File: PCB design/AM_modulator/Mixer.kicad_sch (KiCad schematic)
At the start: 8 parts

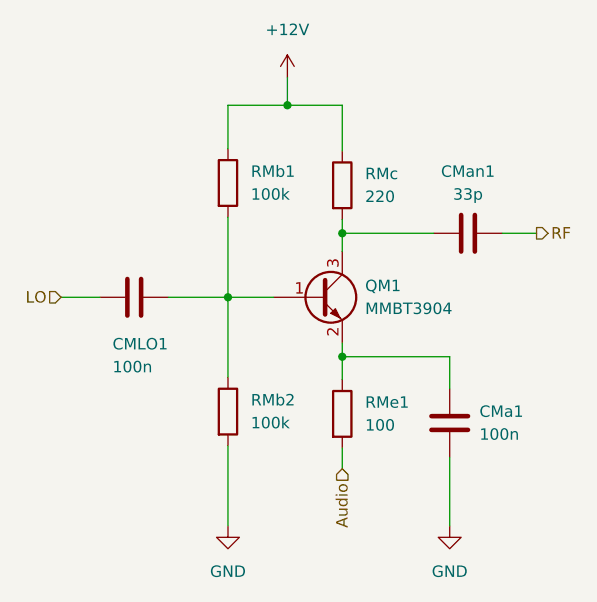
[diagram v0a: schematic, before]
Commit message: Avances placa
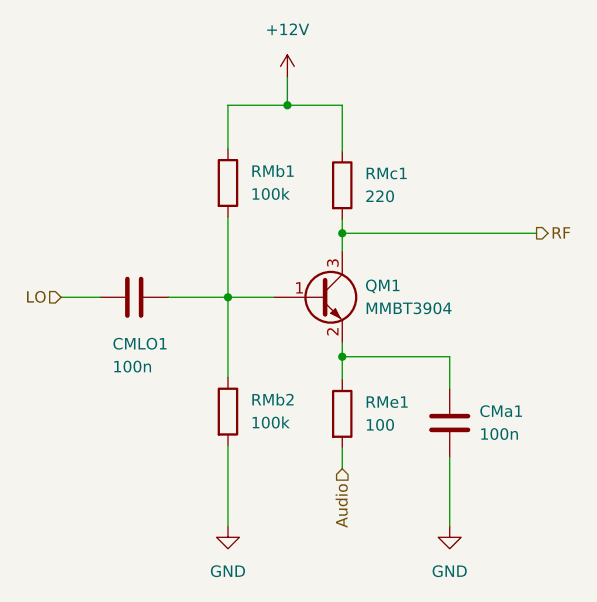
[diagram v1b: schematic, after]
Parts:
- removed CMan1: 33p, Capacitor_SMD:C_0805_2012Metric_Pad1.18x1.45mm_HandSolder, symbol Device:C
- renumbered RMc to RMc1
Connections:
- net RF: now also QM1.3 (C), RMc1.2
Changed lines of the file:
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@@
-    (stroke (width 0) (type default) (color 0 0 0 0))
-  )
-  (wire (pts (xy 156.972 81.788) (xy 160.782 81.788))
     (stroke (width 0) (type default) (color 0 0 0 0))
   )
@@
     (stroke (width 0) (type default) (color 0 0 0 0))
   )
-  (wire (pts (xy 139.192 81.788) (xy 149.352 81.788))
+  (wire (pts (xy 139.192 81.788) (xy 160.782 81.788))
     (stroke (width 0) (type default) (color 0 0 0 0))
   )
@@
     (pin "2")
   )
-  (symbol (lib_id "Device:C") (at 153.162 81.788 90) (unit 1)
-    (in_bom yes) (on_board yes) (fields_autoplaced)
-    (property "Reference" "CMan1" (id 0) (at 153.162 74.93 90))
-    (property "Value" "33p" (id 1) (at 153.162 77.47 90))
-    (property "Footprint" "Capacitor_SMD:C_0805_2012Metric_Pad1.18x1.45mm_HandSolder" (id 2) (at 156.972 80.8228 0)
-      (effects (font (size 1.27 1.27)) hide)
-    )
-    (property "Datasheet" "~" (id 3) (at 153.162 81.788 0)
-      (effects (font (size 1.27 1.27)) hide)
-    )
-    (pin "1")
-    (pin "2")
-  )
   (symbol (lib_id "Device:R") (at 139.192 76.454 0) (unit 1)
     (in_bom yes) (on_board yes) (fields_autoplaced)
-    (property "Reference" "RMc" (id 0) (at 141.732 75.1839 0)
+    (property "Reference" "RMc1" (id 0) (at 141.732 75.1839 0)
       (effects (font (size 1.27 1.27)) (justify left))
     )
